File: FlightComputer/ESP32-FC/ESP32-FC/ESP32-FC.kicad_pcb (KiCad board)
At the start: 2 copper layers, 55 x 40 mm, 50 parts, among them J1 USB_C_Receptacle_USB2.0_16P, J2 Conn_01x02_Pin, J3 Conn_01x04_Pin, J4 Conn_01x03_Pin, J5 Conn_01x03_Pin, SW1 BOOT, SW2 RESET, U1 ESP32-S3-WROOM-1, U2 AP2112K-3.3, U3 ICP-20100, U4 ICM-42670-P, U5 MT3608

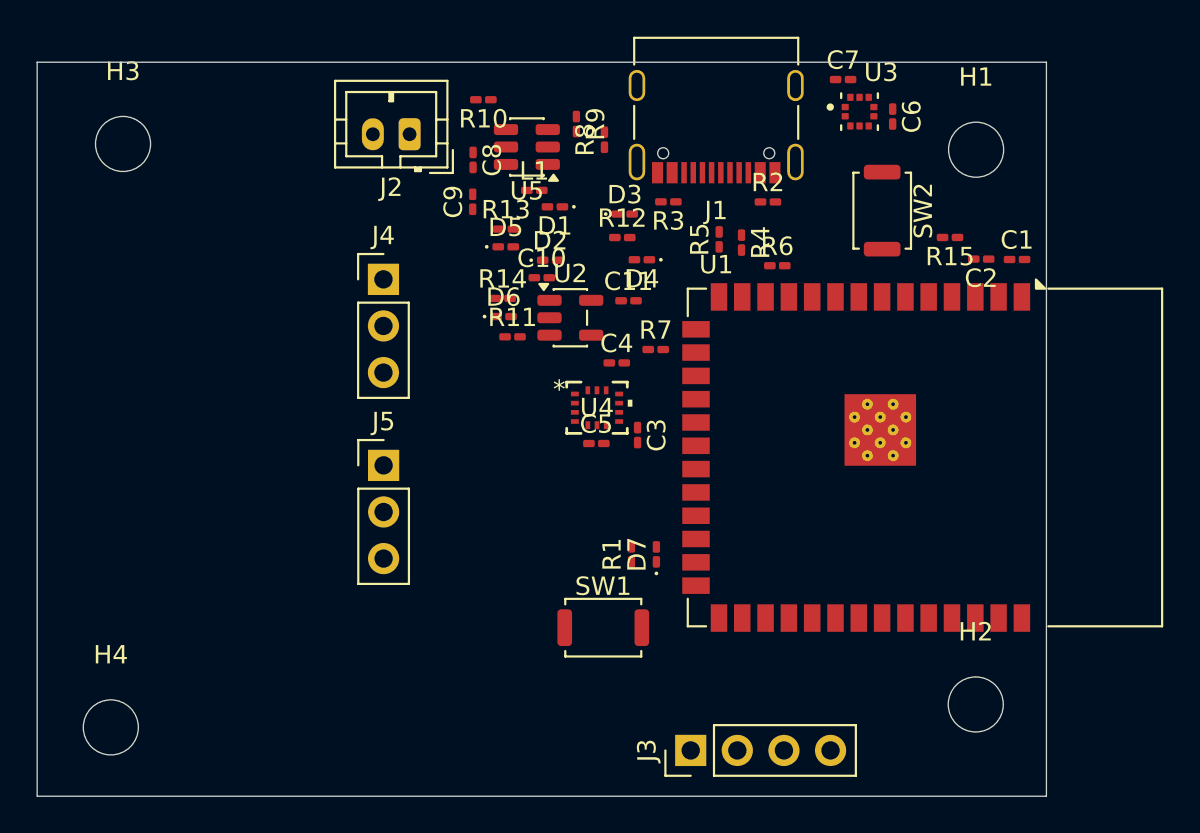
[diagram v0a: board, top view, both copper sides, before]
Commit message: Layout Major
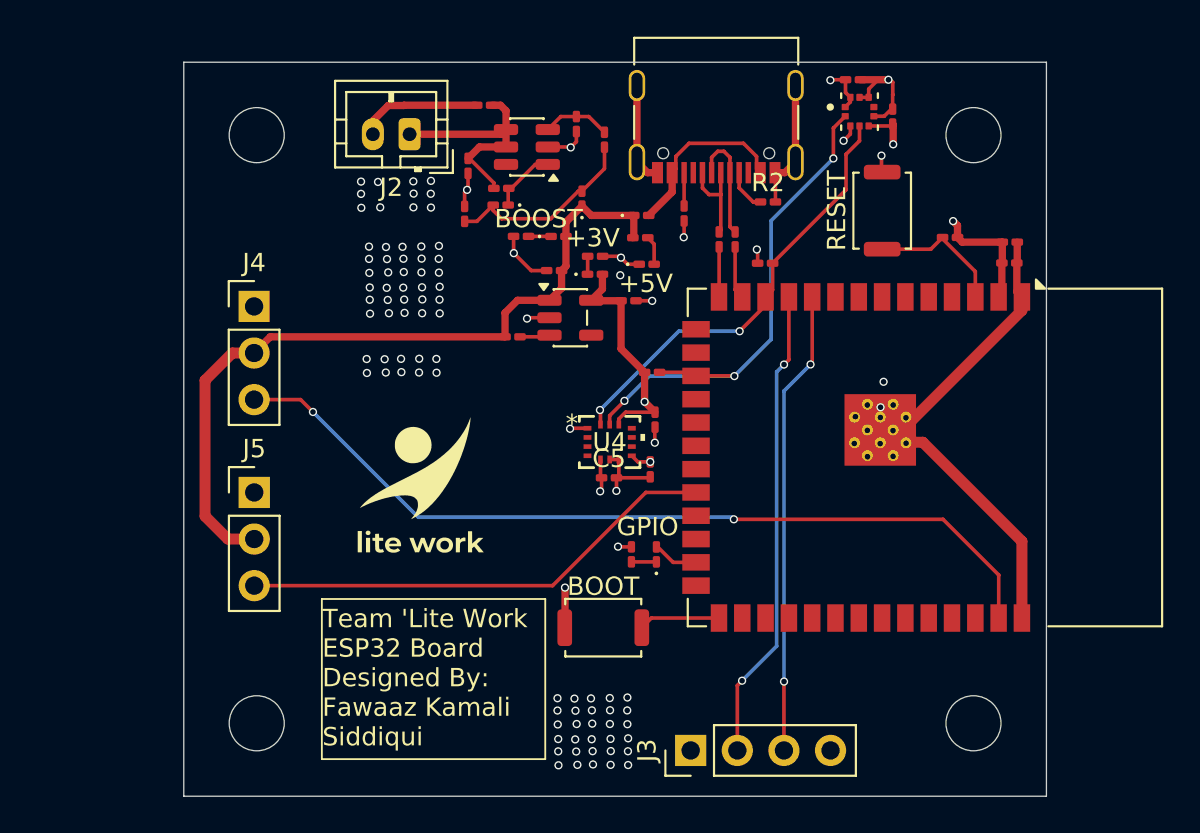
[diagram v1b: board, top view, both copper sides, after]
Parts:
- added G***: LOGO, LOGO, F.Cu at (143.6, 103.1)
- moved H4 7.95 mm to (134.5, 116.0)
- moved H3 7.30 mm to (134.5, 84.0)
- moved J4 7.20 mm to (134.3, 93.3)
- moved J5 7.20 mm to (134.3, 103.4)
- moved R14 5.54 mm to (152.9, 90.6), turned to 180 degrees
- moved +3V 5.49 mm to (152.9, 91.6)
- moved D2 3.78 mm to (152.2, 87.4), turned to 90 degrees
- moved C4 3.73 mm to (156.2, 99.5), turned to -90 degrees
- moved D1 2.96 mm to (147.8, 87.8)
- moved BOOST 2.93 mm to (150.9, 89.5)
- moved C3 1.99 mm to (155.9, 102.2)
- moved C5 1.99 mm to (153.7, 102.6)
- moved U4 1.99 mm to (153.7, 100.7)
- moved L1 1.80 mm to (147.8, 86.9)
- moved C2 1.55 mm to (175.5, 90.9), turned to 0 degrees
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- renumbered D6 to +3V, D4 to +5V, D5 to BOOST, SW1 to BOOT, D7 to GPIO, SW2 to RESET
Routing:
- net +3V3: track 0.00 -> 92.8 mm, vias 0 -> 8
- net GND: track 0.00 -> 79.2 mm, vias 0 -> 110
- net /SERVO1: track 0.00 -> 46.9 mm, vias 0 -> 2
- net +5V: track 0.00 -> 42.1 mm
- net /SCL: track 0.00 -> 29.0 mm, vias 0 -> 3
- net /SERVO2: track 0.00 -> 26.2 mm
- net /ESP_RX: track 0.00 -> 25.9 mm, vias 0 -> 2
- net /ESP_TX: track 0.00 -> 25.4 mm, vias 0 -> 2
- net /SDA: track 0.00 -> 24.1 mm, vias 0 -> 2
- net VBAT: track 0.00 -> 12.8 mm
- net Net-(D1-A): track 0.00 -> 10.8 mm
- net Net-(D3-A): track 0.00 -> 9.78 mm
- net USB_D-: track 0.00 -> 9.17 mm
- net USB_D+: track 0.00 -> 7.98 mm
- net /EN: track 0.00 -> 7.53 mm
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- added copper zone on In1.Cu, net GND
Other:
- board size 55 x 40 mm -> 47 x 40 mm
- copper layers 2 -> 4
- board text added: "Team 'Lite Work ESP32 Board Designed By: Fawaaz Kamali Siddiqui"
